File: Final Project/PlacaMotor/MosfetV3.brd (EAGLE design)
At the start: 42.2 x 37.3 mm, 15 parts, among them IC1 ATTINY44-SSU

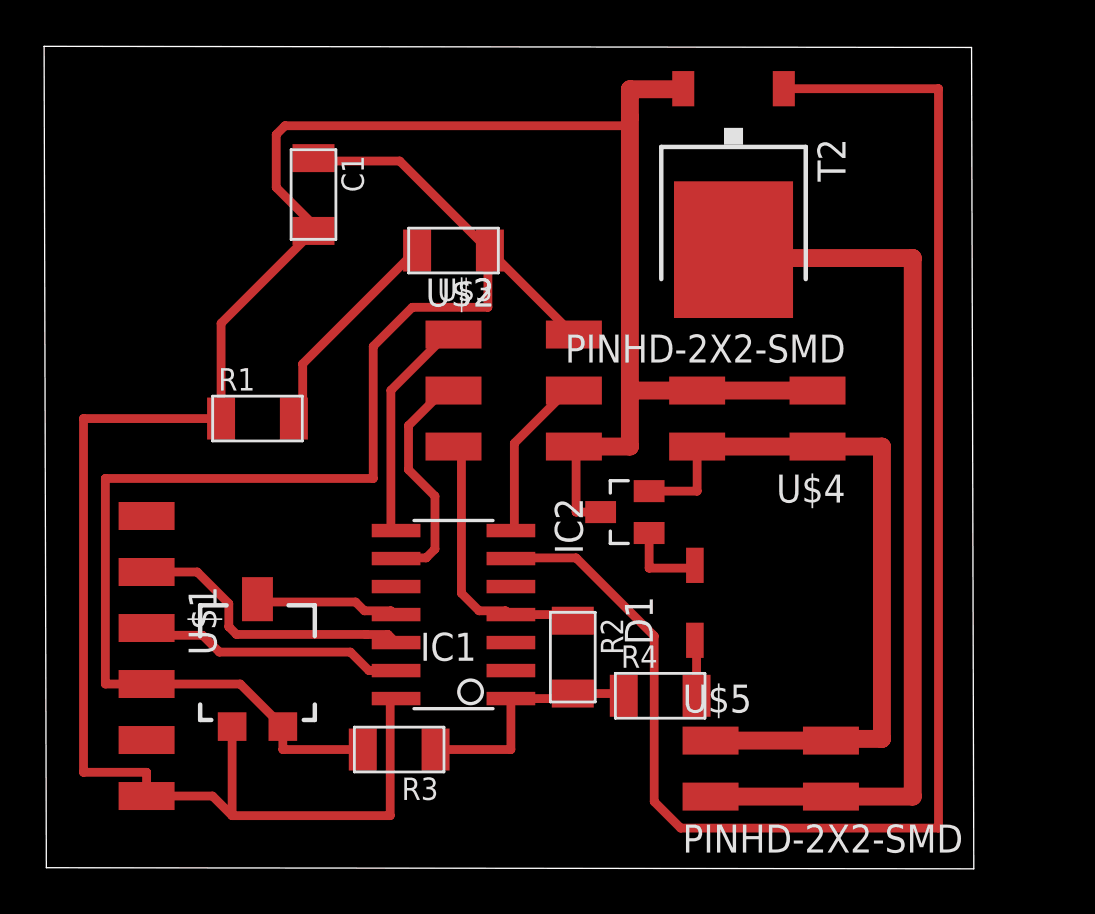
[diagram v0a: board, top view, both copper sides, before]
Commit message: Codigos G
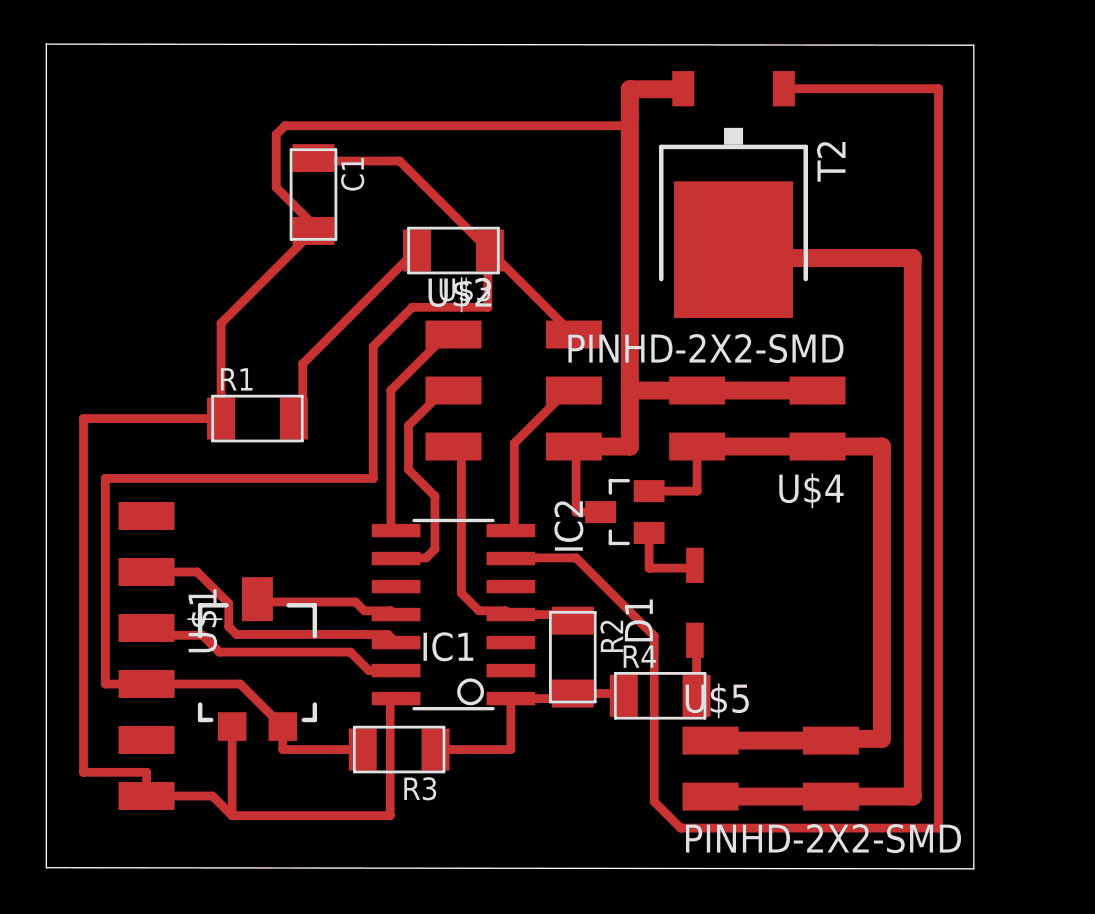
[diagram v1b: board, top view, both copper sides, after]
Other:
- board size 42.2 x 37.3 mm -> 42.1 x 37.4 mm
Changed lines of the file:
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@@
 <plain>
 <wire x1="0.381" y1="-0.1524" x2="42.4436" y2="-0.2032" width="0" layer="20"/>
-<wire x1="42.4436" y1="-0.2032" x2="42.342" y2="37.0486" width="0" layer="20"/>
-<wire x1="42.342" y1="37.0486" x2="0.2794" y2="37.0994" width="0" layer="20"/>
-<wire x1="0.2794" y1="37.0994" x2="0.381" y2="-0.1524" width="0" layer="20"/>
+<wire x1="42.4436" y1="-0.2032" x2="42.4436" y2="37.1502" width="0" layer="20"/>
+<wire x1="42.4436" y1="37.1502" x2="0.381" y2="37.201" width="0" layer="20"/>
+<wire x1="0.381" y1="37.201" x2="0.381" y2="-0.1524" width="0" layer="20"/>
 </plain>
 <attributes>
